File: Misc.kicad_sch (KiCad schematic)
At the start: 18 parts, among them J3 Conn_02x08_Odd_Even, J4 BM04B-SURS-TFLFSN, J5 Conn_02x04_Odd_Even, J6 Conn_02x04_Odd_Even, J7 Conn_01x05, J8 Conn_01x04, U5 SN65HVD232QDRQ1

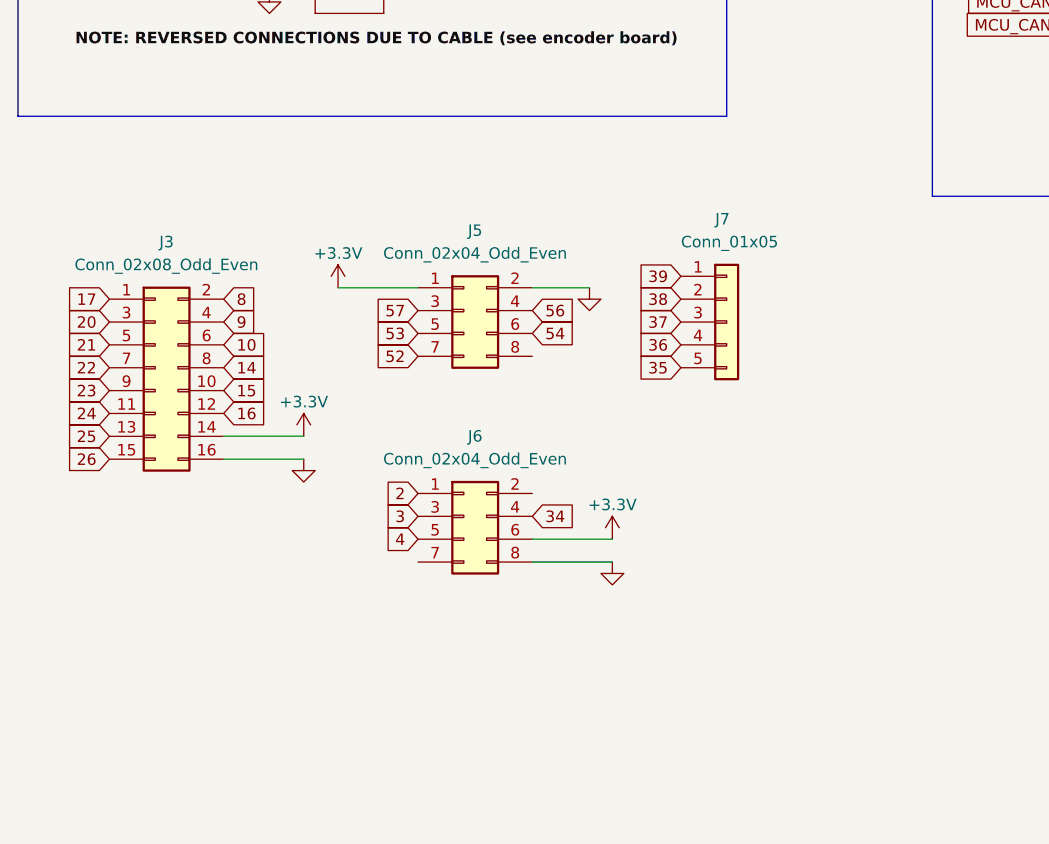
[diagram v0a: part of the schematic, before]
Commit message: stuff
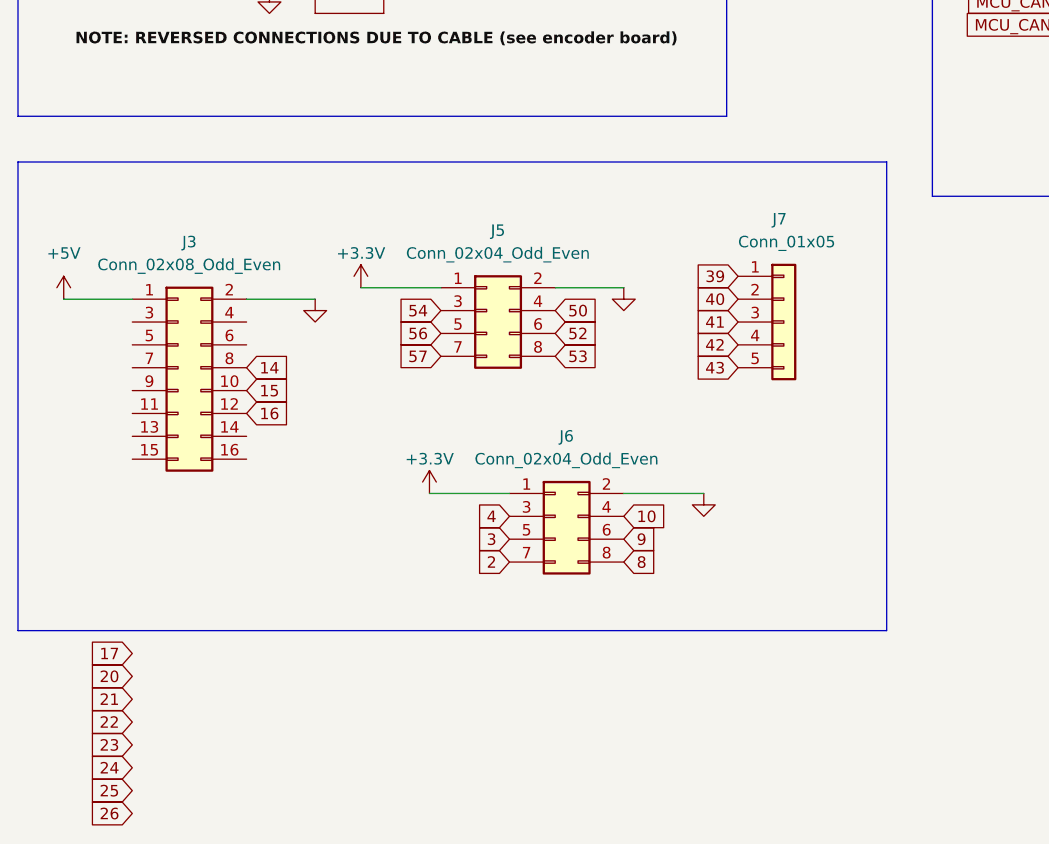
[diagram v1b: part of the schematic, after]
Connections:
- net 34 is gone; now on net 10: J6.4 (Pin_4)
- net +3V3: now also J6.1 (Pin_1); no longer J3.14 (Pin_14), J6.6 (Pin_6)
- net 10: no longer J3.6 (Pin_6)
- net 17: no longer J3.1 (Pin_1)
- net 2: now also J6.7 (Pin_7); no longer J6.1 (Pin_1)
- net 20: no longer J3.3 (Pin_3)
- net 21: no longer J3.5 (Pin_5)
- net 22: no longer J3.7 (Pin_7)
- net 23: no longer J3.9 (Pin_9)
- net 24: no longer J3.11 (Pin_11)
- net 25: no longer J3.13 (Pin_13)
- net 26: no longer J3.15 (Pin_15)
- net 3: now also J6.5 (Pin_5); no longer J6.3 (Pin_3)
- net 4: now also J6.3 (Pin_3); no longer J6.5 (Pin_5)
- net 52: now also J5.6 (Pin_6); no longer J5.7 (Pin_7)
- net 53: now also J5.8 (Pin_8); no longer J5.5 (Pin_5)
- net 54: now also J5.3 (Pin_3); no longer J5.6 (Pin_6)
- net 56: now also J5.5 (Pin_5); no longer J5.4 (Pin_4)
- net 57: now also J5.7 (Pin_7); no longer J5.3 (Pin_3)
- net 8: now also J6.8 (Pin_8); no longer J3.2 (Pin_2)
- net 9: now also J6.6 (Pin_6); no longer J3.4 (Pin_4)
- net GND: now also J3.2 (Pin_2), J6.2 (Pin_2); no longer J3.16 (Pin_16), J6.8 (Pin_8)
- net 35 renamed 43
- net 36 renamed 42
- net 37 renamed 41
- net 38 renamed 40
- new net +5V: J3.1 (Pin_1)
- new net 50: J5.4 (Pin_4)
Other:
- moved on the sheet: J3, J5, J6, J7
